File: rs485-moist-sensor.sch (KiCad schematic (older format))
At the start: 26 parts, among them IC1 ATTINY441-MU, P1 CONN_02X03, P2 CONN_01X04, U1 SP3481EN, X1 16MHz

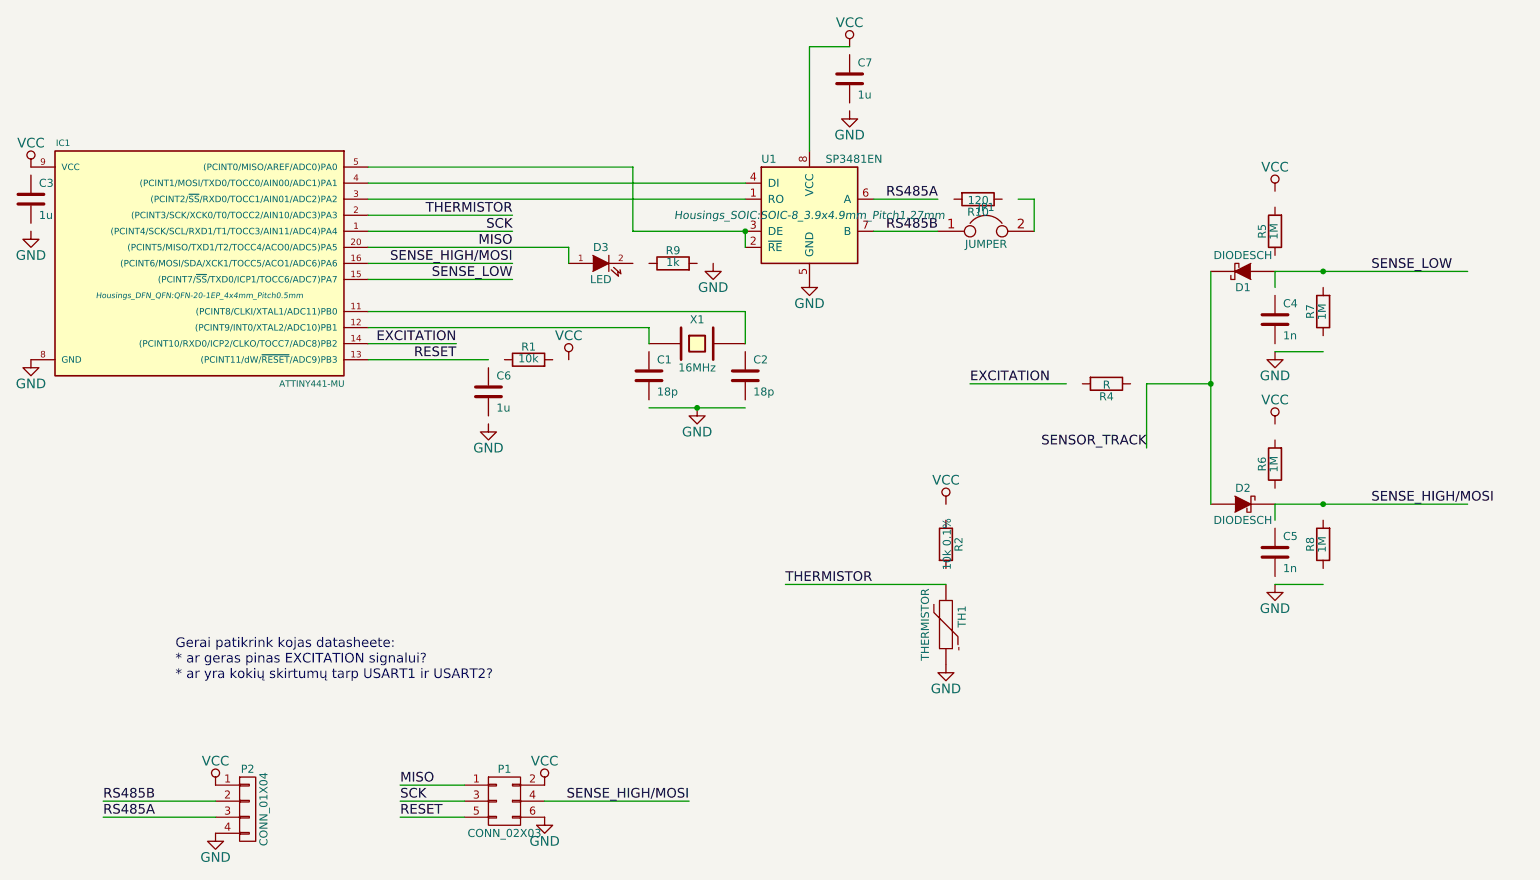
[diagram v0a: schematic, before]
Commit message: Some most recent changes
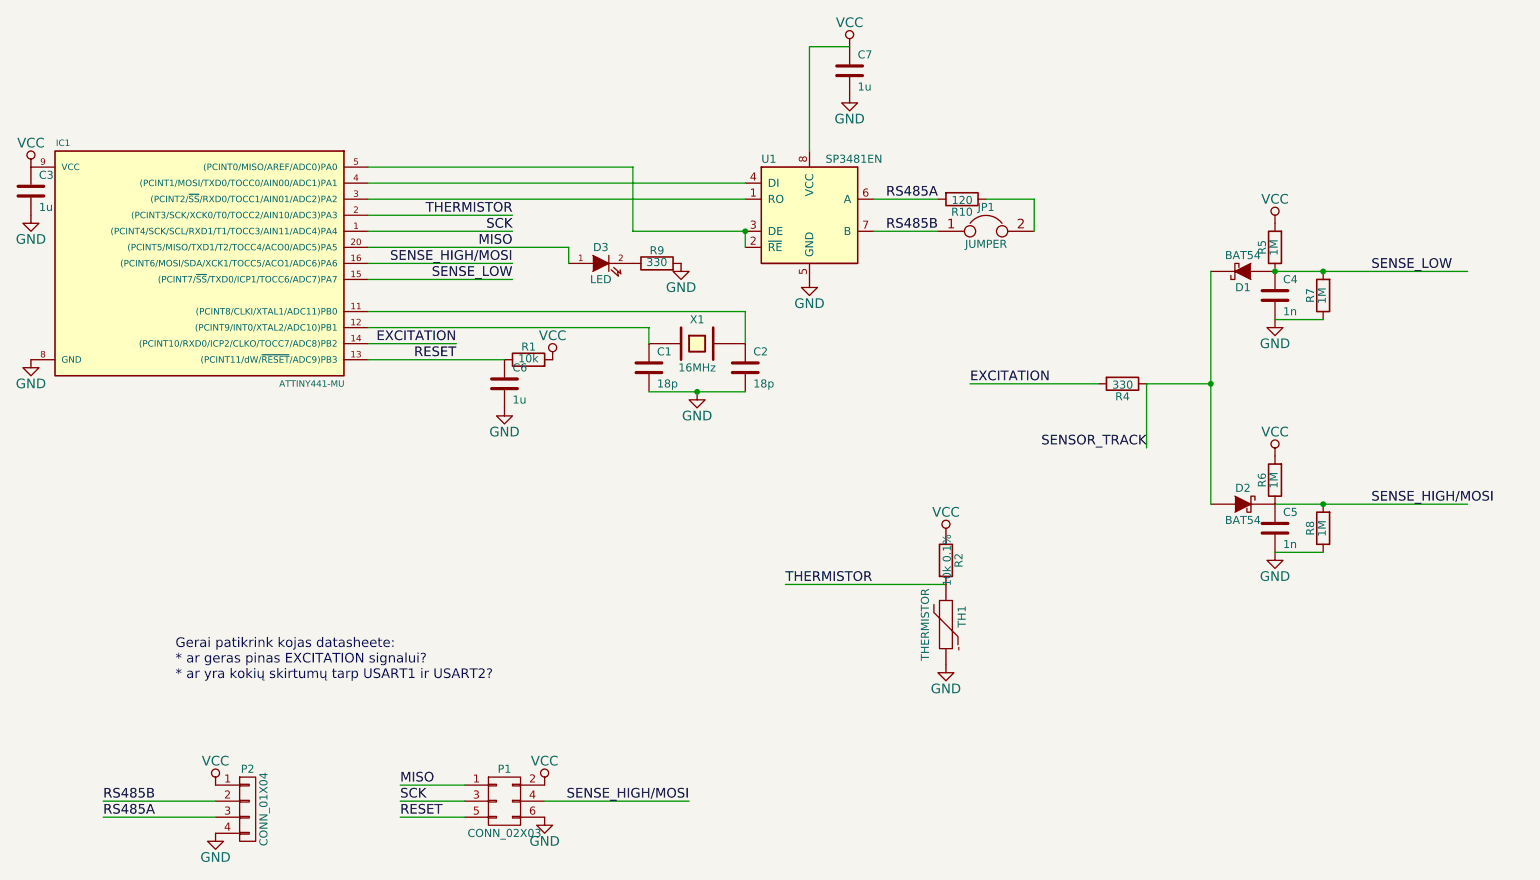
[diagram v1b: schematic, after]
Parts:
- D1, D2: value DIODESCH -> BAT54
- R4: value R -> 330
- R9: value 1k -> 330
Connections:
- wire segments 42 -> 40
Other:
- moved on the sheet: C1, C2, C3, C4, C5, C6, C7, R10, R2, R4, R5, R6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
